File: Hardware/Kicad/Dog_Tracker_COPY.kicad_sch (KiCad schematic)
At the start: 20 parts, among them IC1 M4 Feather, U1 ADP160AUJZ-1.8-R7, U2 SX1280IMLTRT, U3 Origin_GPS1510, U4 NFA18SL407V1A45L, U5 SN74AUP1T97, U6 LSM6DSO32

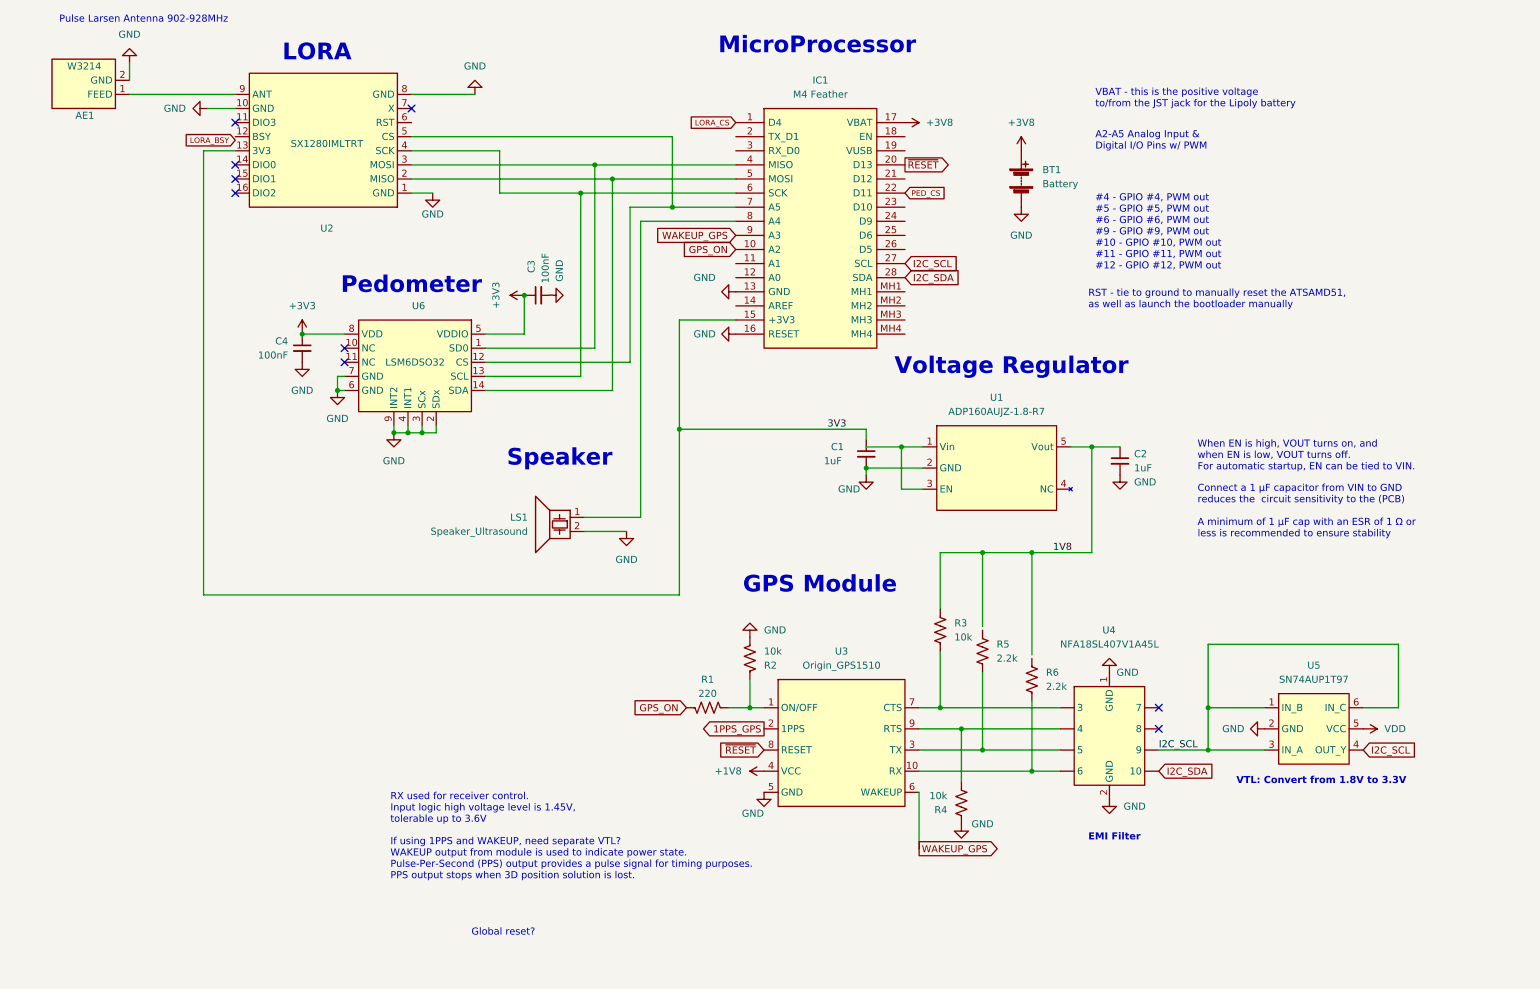
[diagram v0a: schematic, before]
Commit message: 'wire the schematic'
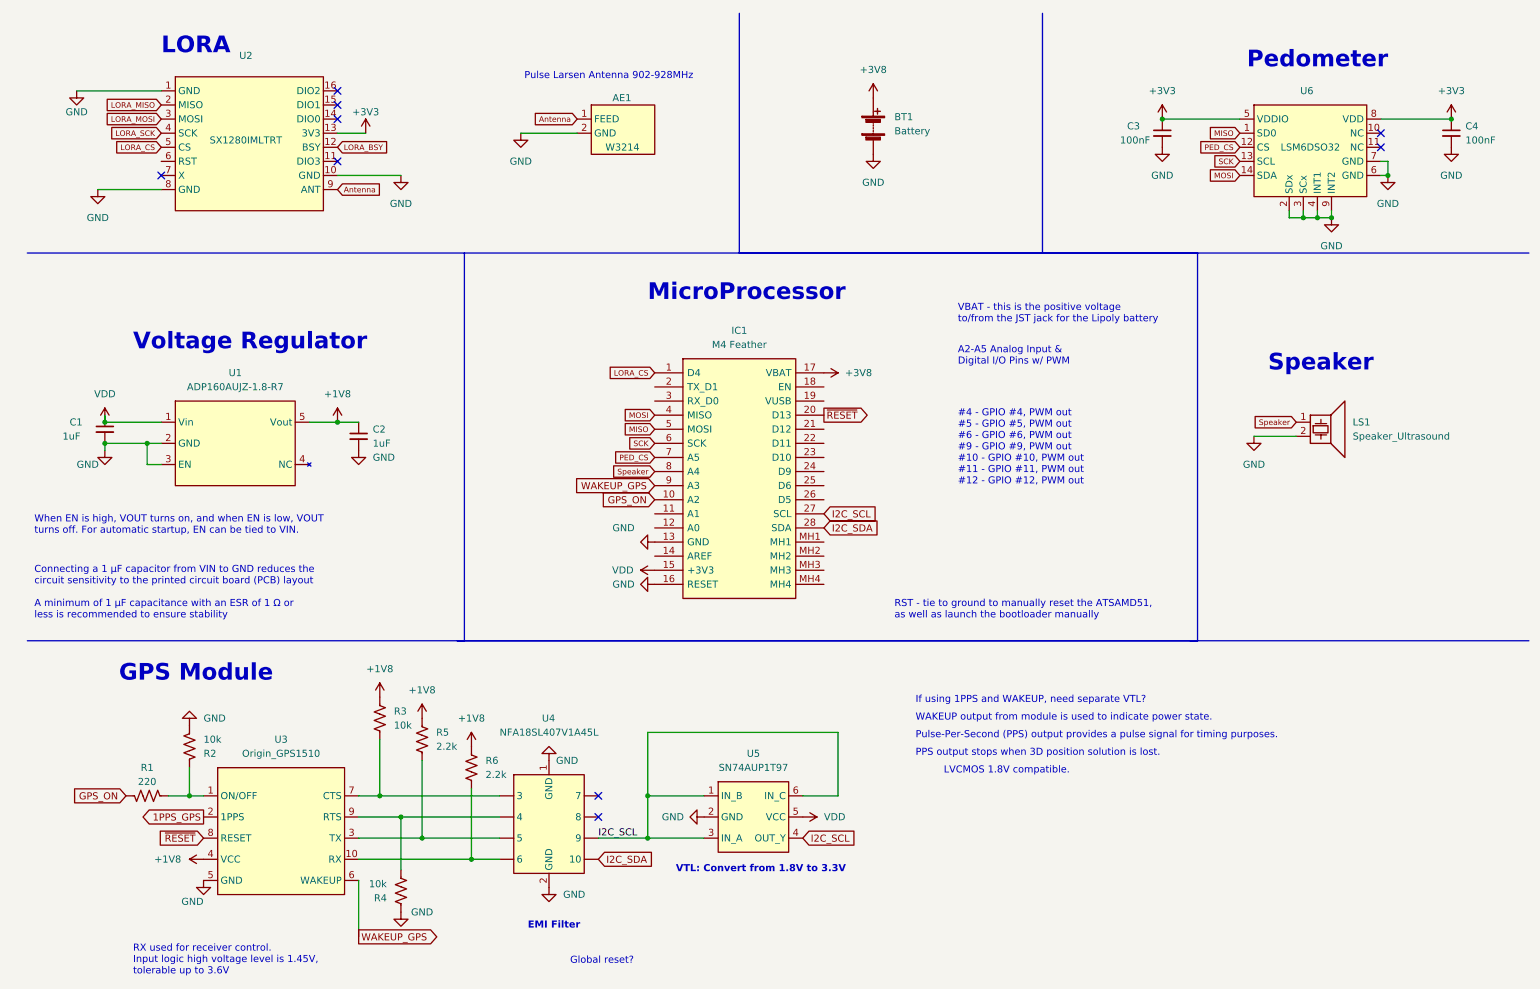
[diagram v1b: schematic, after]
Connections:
- net 1V8 is gone; now on net +1V8: C2.1, R3.2, U1.5 (Vout)
- net +1V8: now also R5.2, R6.2
- net +3V3: now also U2.13 (3V3)
- net GND: now also U1.3 (EN)
- net LORA_BSY: now also U2.12 (BSY)
- net LORA_CS: now also U2.5 (CS)
- net PED_CS: now also IC1.7 (A5), U6.12 (CS); no longer IC1.22 (D11)
- net VDD: now also C1.1, IC1.15 (+3V3), U1.1 (Vin)
- net Speaker: now reaches IC1.8 (A4), LS1.1
- net SCK: now reaches IC1.6 (SCK), U6.13 (SCL)
- net SCK: no longer U2.4 (SCK)
- net Antenna: now reaches AE1.1 (FEED), U2.9 (ANT)
- removed net 3V3: C1.1, IC1.15 (+3V3), U2.13 (3V3)
- new net LORA_MISO: U2.2 (MISO)
- new net LORA_MOSI: U2.3 (MOSI)
- new net LORA_SCK: U2.4 (SCK)
- new net MISO: IC1.5 (MOSI), U6.1 (SD0)
- new net MOSI: IC1.4 (MISO), U6.14 (SDA)
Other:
- note added: "Connecting a 1 μF capacitor from VIN to GND reduces the circuit sensitivity to the printed circuit board (PCB) layout A minimum of 1 μF capacitance with an ESR of 1 Ω or less is recommended to ensure stability"
- note added: "If using 1PPS and WAKEUP, need separate VTL?"
- note added: "LVCMOS 1.8V compatible."
- note added: "PPS output stops when 3D position solution is lost."
- note added: "Pulse-Per-Second (PPS) output provides a pulse signal for timing purposes."
- note added: "WAKEUP output from module is used to indicate power state."
- note removed: "Connect a 1 μF capacitor from VIN to GND reduces the circuit sensitivity to the (PCB) A minimum of 1 μF cap with an ESR of 1 Ω or less is recommended to ensure stability"
- note removed: "If using 1PPS and WAKEUP, need separate VTL? WAKEUP output from module is used to indicate power state. Pulse-Per-Second (PPS) output provides a pulse signal for timing purposes. PPS output stops when 3D position solution is lost."
- moved on the sheet: AE1, BT1, C1, C2, C3, C4, IC1, LS1, R1, R2, R3, R4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
